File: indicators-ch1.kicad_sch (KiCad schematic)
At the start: 2 parts, among them U10 74HC123

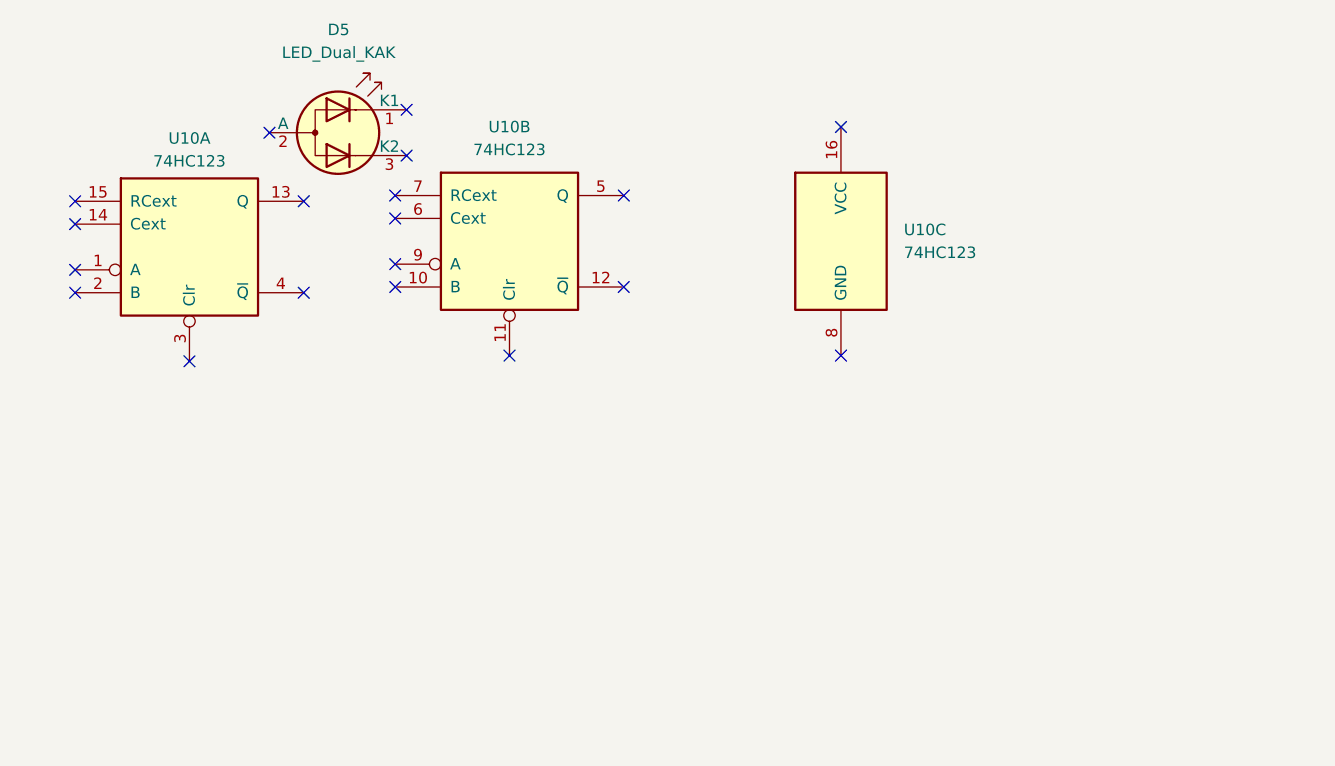
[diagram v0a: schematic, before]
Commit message: Flush
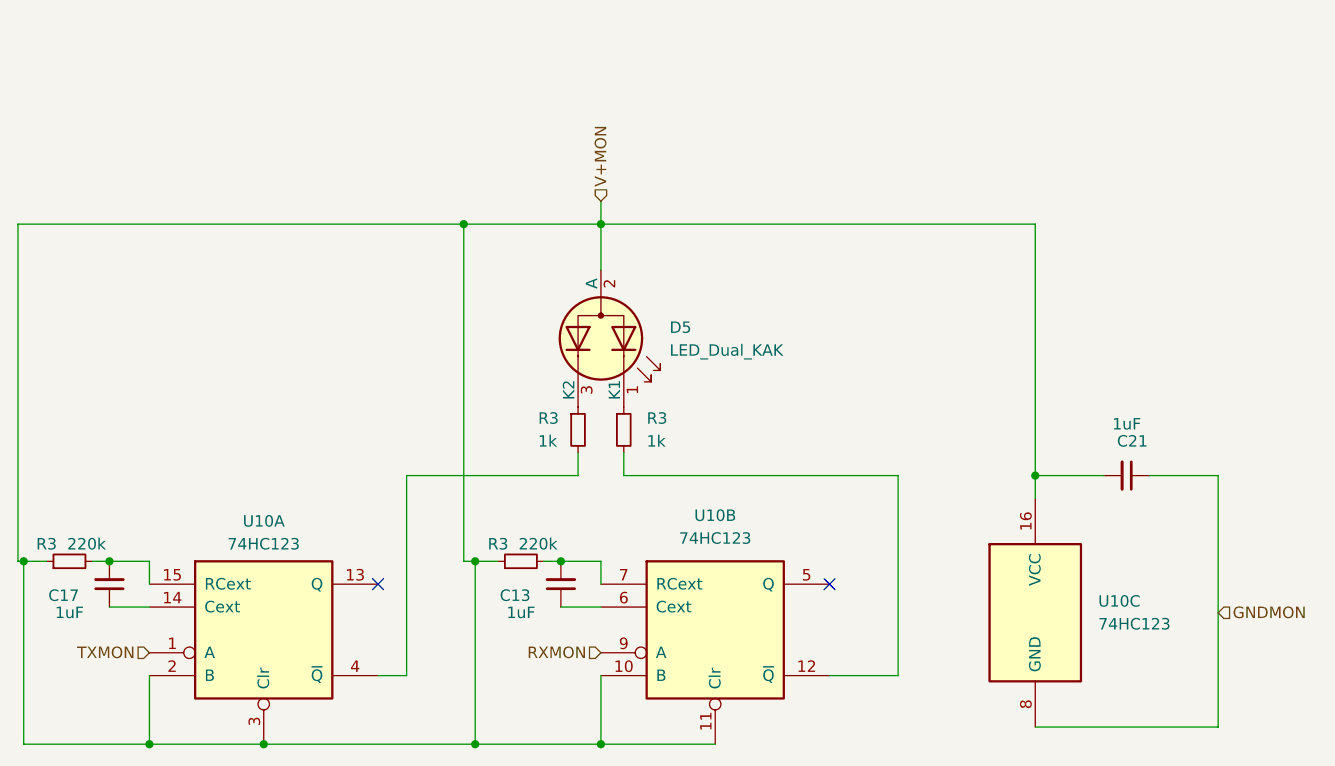
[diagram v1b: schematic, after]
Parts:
- added C13, C17, C21: 1uF, Capacitor_SMD:C_0805_2012Metric_Pad1.18x1.45mm_HandSolder, symbol Device:C_Small
- added R3 (x2): 1k, Resistor_SMD:R_0805_2012Metric_Pad1.20x1.40mm_HandSolder, symbol Device:R_Small
- added R3 (x2): 220k, Resistor_SMD:R_0805_2012Metric_Pad1.20x1.40mm_HandSolder, symbol Device:R_Small
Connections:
- net V+MON: now reaches U10.16 (VCC)
- net V+MON: now also D5.2 (A), U10.10 (B), U10.11 (Clr), U10.2 (B), U10.3 (Clr), C21.2, R3.1, R3.1
- net GNDMON: now reaches U10.8 (GND)
- net GNDMON: now also C21.1
- net at D5.1 (K1): now also R3.1
- net at D5.3 (K2): now also R3.1
- net TXMON: now reaches U10.1 (A)
- net at U10.14 (Cext): now also C17.1
- net at U10.15 (RCext): now also C17.2, R3.2
- net at U10.4 (~{Q}): now also R3.2
- net at U10.12 (~{Q}): now also R3.2
- net at U10.6 (Cext): now also C13.1
- net at U10.7 (RCext): now also C13.2, R3.2
- net RXMON: now reaches U10.9 (A)
- no-connect marks 19 -> 2
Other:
- moved on the sheet: D5, U10A, U10B, U10C
